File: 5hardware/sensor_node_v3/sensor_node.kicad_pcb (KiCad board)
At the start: 2 copper layers, 28 parts, among them J1 Conn_01x03, J3 Conn_01x29, SW2 SW_DIP_x04, SW3 SW_Push, SW4 SW_DIP_x04, SW5 RotaryEncoder, SW6 SW_Push, U1 MCP1700x-330xxTO, U7 CH32V003F4P6, U8 ESP32-WROOM-32D

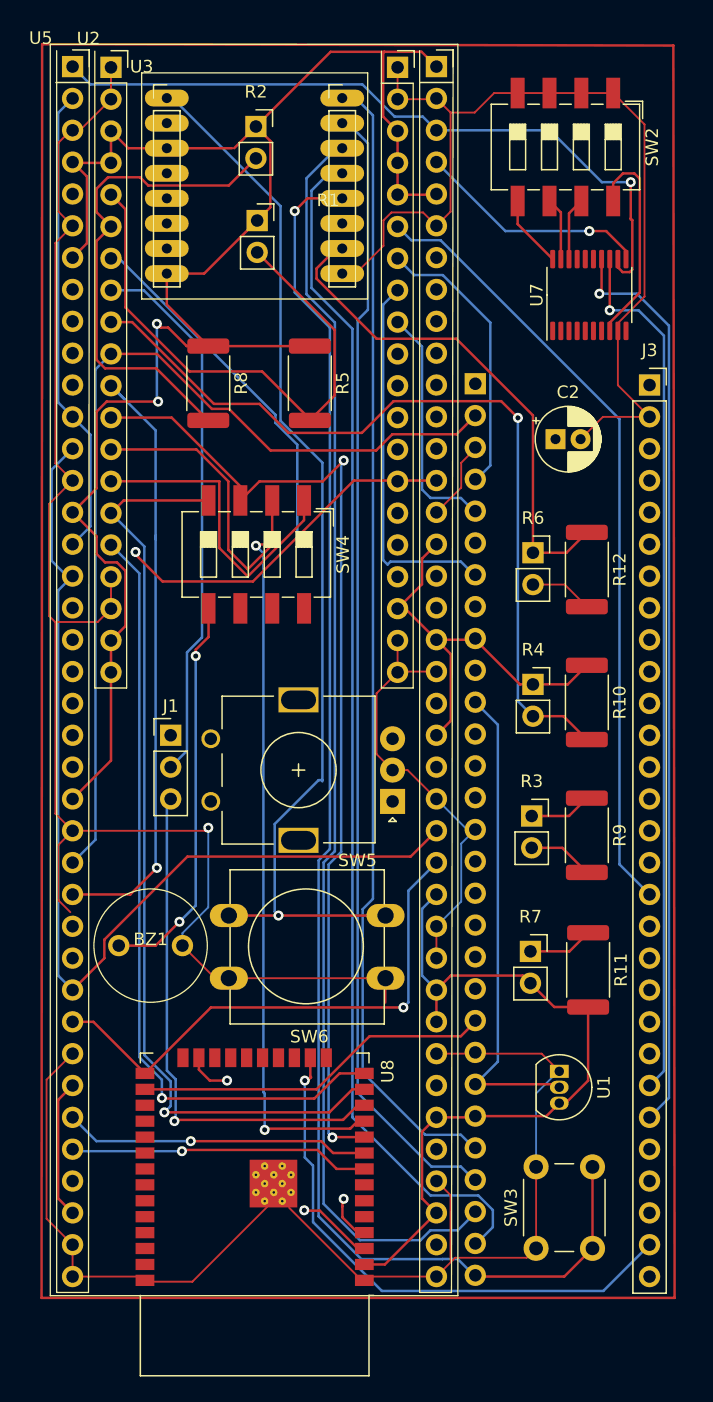
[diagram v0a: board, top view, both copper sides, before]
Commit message: updating pcb design.
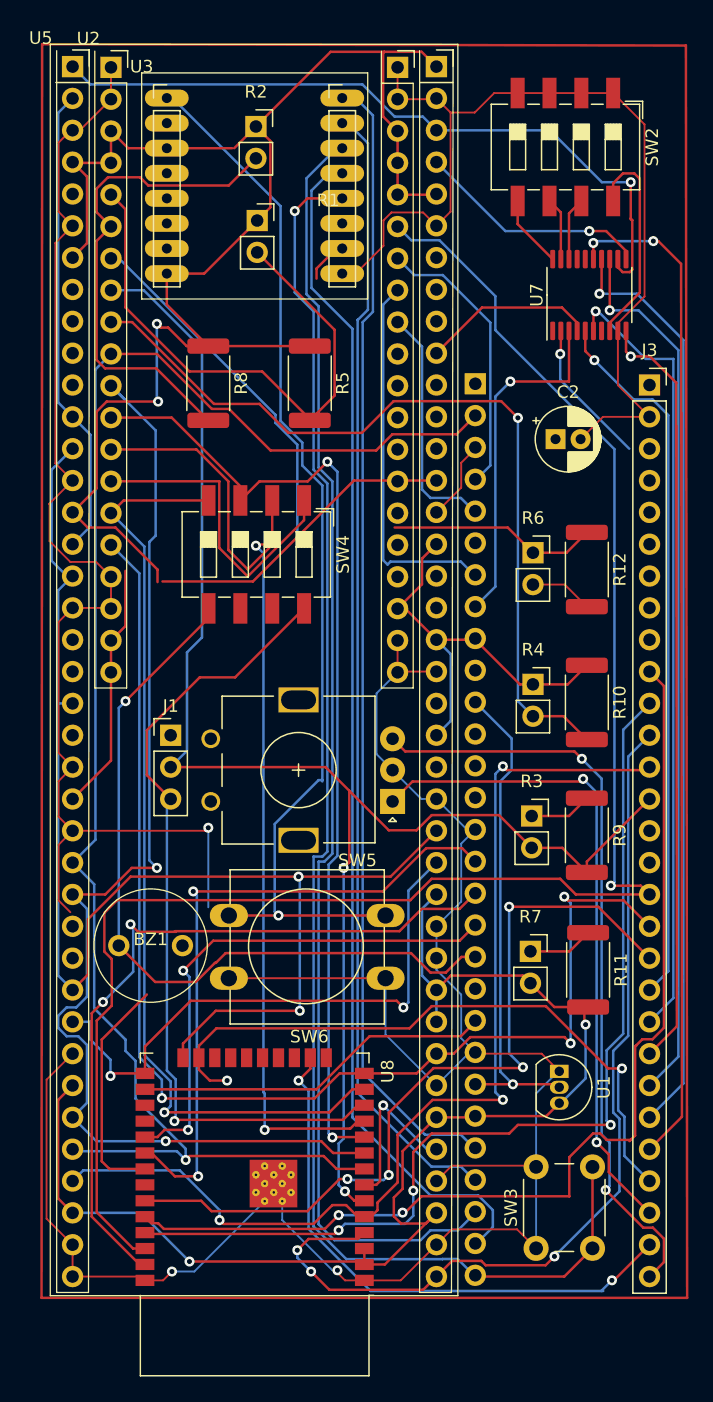
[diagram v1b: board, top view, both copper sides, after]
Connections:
- C2 pad 1: +3.3V -> EN
- J3 pad 1: +3.3V -> EN
- J3 pad 10: unconnected-(J3-Pin_10-Pad10) -> RX (3)
- J3 pad 11: unconnected-(J3-Pin_11-Pad11) -> TX (1)
- J3 pad 19: FREE (21) -> AUD (21)
- J3 pad 3: unconnected-(J3-Pin_3-Pad3) -> OD1
- J3 pad 5: unconnected-(J3-Pin_5-Pad5) -> OD0
- J3 pad 9: unconnected-(J3-Pin_9-Pad9) -> OD2
- R1 pad 1: +3.3V -> EN
- R10 pad 1: +3.3V -> EN
- R11 pad 2: +3.3V -> EN
- R2 pad 1: +3.3V -> EN
- R2 pad 2: IO_k39 -> IO_39
- R3 pad 1: +3.3V -> EN
- R4 pad 1: +3.3V -> EN
- R5 pad 1: +3.3V -> EN
- R7 pad 2: +3.3V -> EN
- R8 pad 1: +3.3V -> EN
- R8 pad 2: IO_k39 -> IO_39
- R9 pad 1: +3.3V -> EN
- SW4 pad 1: BCLK -> OD3 (27)
- SW4 pad 8: OD3 -> BCLK
- U1 pad 3: +3.3V -> EN
- U2 pad 14: BCLK -> OD3 (27)
- U2 pad 19: +3.3V -> EN
- U2 pad 20: +3.3V -> EN
- U2 pad 23: +3.3V -> EN
- U2 pad 24: +3.3V -> EN
- U2 pad 25: +3.3V -> EN
- U2 pad 3: +3.3V -> EN
- U2 pad 38: +3.3V -> EN
- U2 pad 4: +3.3V -> EN
- U2 pad 6: IO_k39 -> IO_39
- U3 pad 3: +3.3V -> EN
- U3 pad 8: +3.3V -> EN
- U4 pad 24: +3.3V -> EN
- U4 pad 3: GND -> EN
- U4 pad 4: MISO (19) -> GND
- U4 pad 5: SCK (18) -> MISO (19)
- U4 pad 6: SDA (33) -> SCK (18)
- U4 pad 9: +3.3V -> EN
- U5 pad 1: SDA1 (4) -> SDA1 (2)
- U5 pad 10: unconnected-(U5-A+-Pad10) -> AUD (21)
- U5 pad 13: SDA1 (4) -> SDA1 (2)
- U5 pad 15: +3.3V -> EN
- U5 pad 17: SDA1 (4) -> SDA1 (2)
- U5 pad 18: unconnected-(U5-_RES-Pad18) -> GND
- U5 pad 19: unconnected-(U5-_DC-Pad19) -> EN
- U5 pad 21: unconnected-(U5-_LED-Pad21) -> SDA1 (2)
- U5 pad 22: unconnected-(U5-x-Pad22) -> SCL1 (0)
- U5 pad 23: unconnected-(U5-x-Pad23) -> GND
- U5 pad 24: +3.3V -> EN
- U5 pad 30: SDA1 (4) -> SDA1 (2)
- U5 pad 33: +3.3V -> EN
- U5 pad 36: unconnected-(U5-PIR-Pad36) -> IO_39
- U5 pad 37: +3.3V -> EN
- U5 pad 4: +3.3V -> EN
- U5 pad 40: +3.3V -> EN
- U5 pad 42: SDA1 (4) -> SDA1 (2)
- U5 pad 44: +3.3V -> EN
- U5 pad 48: unconnected-(U5-DIN-Pad48) -> IO_34
- U5 pad 5: AUD -> unconnected-(U5-_OUT-Pad5)
- U5 pad 51: unconnected-(U5-x-Pad51) -> TX2 (16)
- U5 pad 52: SDA1 (4) -> SDA1 (2)
- U5 pad 55: +3.3V -> EN
- U5 pad 56: unconnected-(U5-x-Pad56) -> RX2 (17)
- U5 pad 58: +3.3V -> EN
- U5 pad 61: +3.3V -> EN
- U5 pad 62: unconnected-(U5-WS28-Pad62) -> WLED (12)
- U5 pad 64: SDA1 (4) -> SDA1 (2)
- U5 pad 66: +3.3V -> EN
- U5 pad 69: +3.3V -> EN
- U5 pad 7: +3.3V -> EN
- U5 pad 70: +3.3V -> EN
- U5 pad 71: GND -> WLED (12)
- U5 pad 72: unconnected-(U5-OUT-Pad72) -> GND
- U5 pad 73: +3.3V -> EN
- U5 pad 74: unconnected-(U5-OUT-Pad74) -> IO_35
- U5 pad 76: +3.3V -> EN
- U5 pad 77: unconnected-(U5-OUT-Pad77) -> GND
- U5 pad 78: GND -> IO_36
- U5 pad 9: unconnected-(U5-A--Pad9) -> GND
- U7 pad 12: SDA1 (4) -> SDA1 (2)
- U7 pad 4: OD3 -> BCLK
- U7 pad 7: +3.3V -> EN
- U8 pad 12: BCLK -> OD3 (27)
- U8 pad 2: +3.3V -> EN
- U8 pad 33: FREE (21) -> AUD (21)
- U8 pad 34: RX -> RX (3)
- U8 pad 35: TX -> TX (1)
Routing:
- net EN: track 35.6 -> 317.3 mm, vias 1 -> 4
- net +3.3V: track 253.2 -> 0.00 mm, vias 2 -> 0
- net SDA1 (2): track 0.00 -> 164.5 mm, vias 0 -> 3
- net SDA1 (4): track 139.3 -> 0.00 mm, vias 1 -> 0
- net IO_39: track 0.00 -> 123.2 mm, vias 0 -> 3
- net RX (3): track 0.00 -> 84.0 mm, vias 0 -> 2
- net Net-(J3-Pin_25): track 0.00 -> 80.8 mm, vias 0 -> 2
- net TX (1): track 0.00 -> 78.9 mm, vias 0 -> 3
- net LED (22): track 63.0 -> 139.4 mm, vias 0 -> 1
- net IO_34: track 48.8 -> 123.6 mm, vias 0 -> 2
- net IO_36: track 48.5 -> 119.7 mm, vias 1 -> 3
- net AUD (21): track 0.00 -> 64.4 mm, vias 0 -> 4
- net Net-(J3-Pin_21): track 0.00 -> 63.1 mm, vias 0 -> 1
- net Net-(J3-Pin_22): track 0.00 -> 61.1 mm, vias 0 -> 1
- net Net-(J3-Pin_29): track 0.00 -> 61.0 mm, vias 0 -> 2
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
